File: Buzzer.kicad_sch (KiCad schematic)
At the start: 6 parts, among them J7 BuzzConn, Q1 PSMN8R5-40MSDX

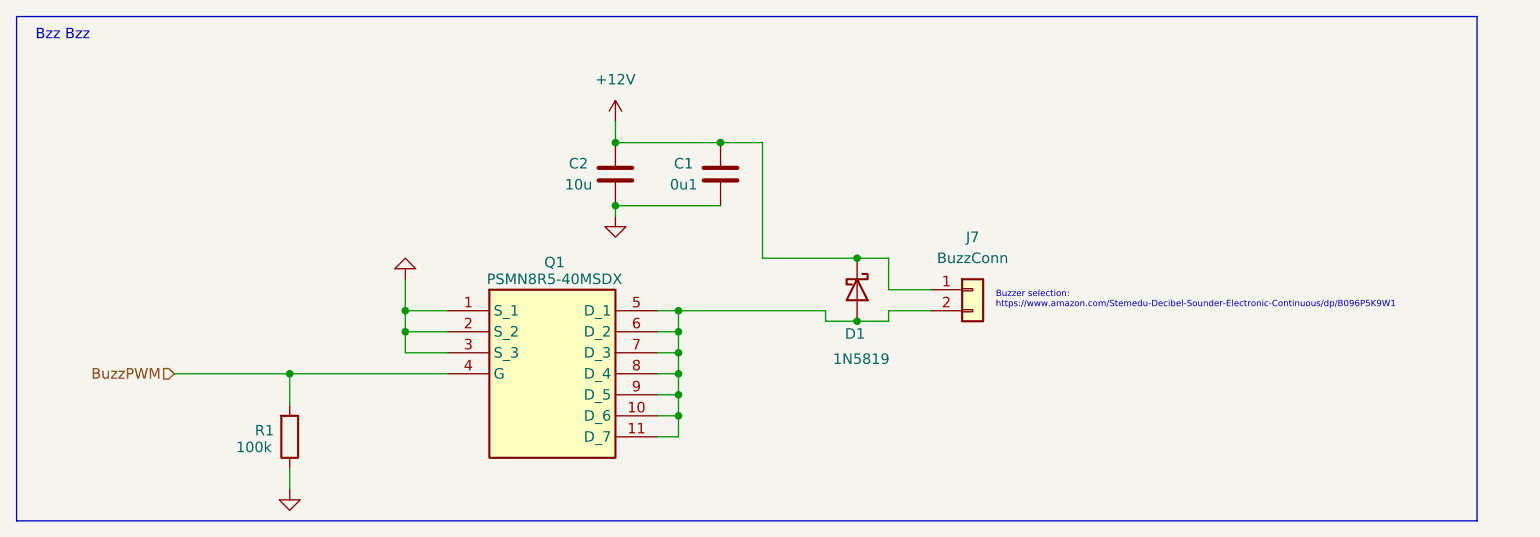
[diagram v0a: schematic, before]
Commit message: RevA9 for review
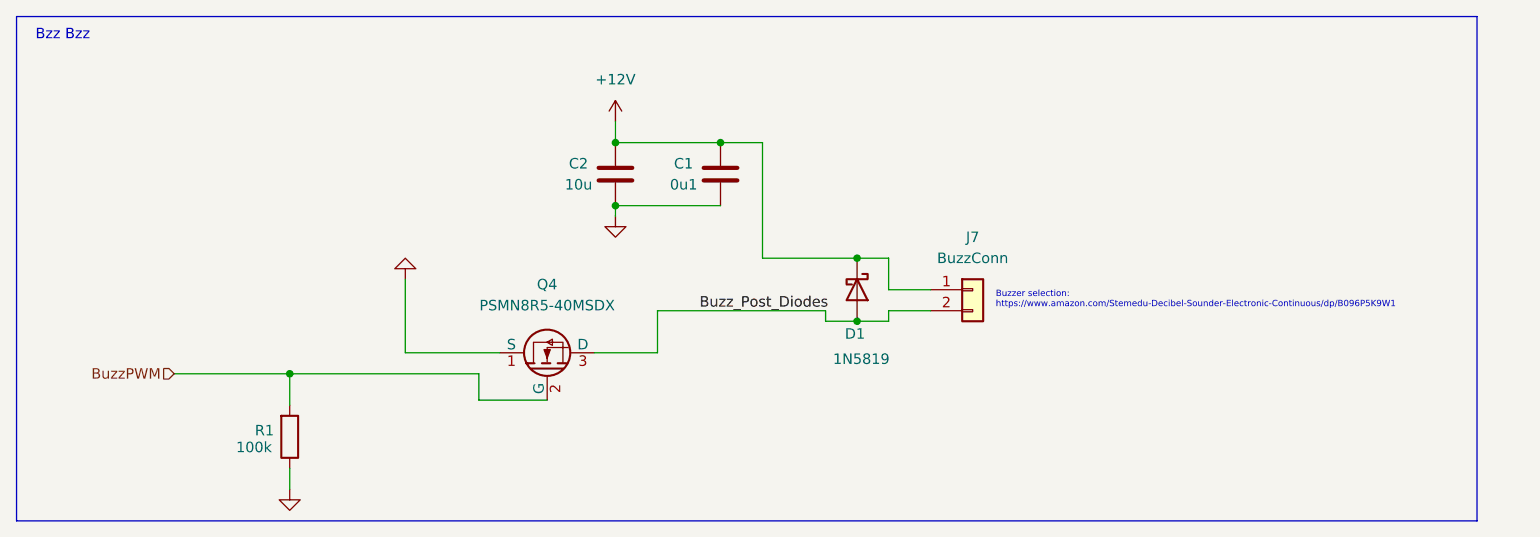
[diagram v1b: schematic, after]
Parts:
- removed Q1: PSMN8R5-40MSDX, UTSVT_Power:PSMN8R5-40MSDX, symbol utsvt_power:PSMN8R5-40MSDX
- added Q4: PSMN8R5-40MSDX, UTSVT_Power:PSMN8R5-40MSDX, symbol utsvt_power:PSMN8R5-40MSDX
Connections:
- net BuzzPWM: now also Q4.2 (G)
- net GND: now also Q4.1 (S)
- net Buzz_Post_Diodes: now reaches D1.2 (A), J7.2 (Pin_2)
- net Buzz_Post_Diodes: now also Q4.3 (D)
